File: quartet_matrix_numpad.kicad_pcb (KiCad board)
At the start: 2 copper layers, 100 x 100 mm, 62 parts, among them J2 QUARTET_RECV, SW1 Rotary_Encoder_Switch, U1 MCP23017_SS, U2 IS31FL3731-SA

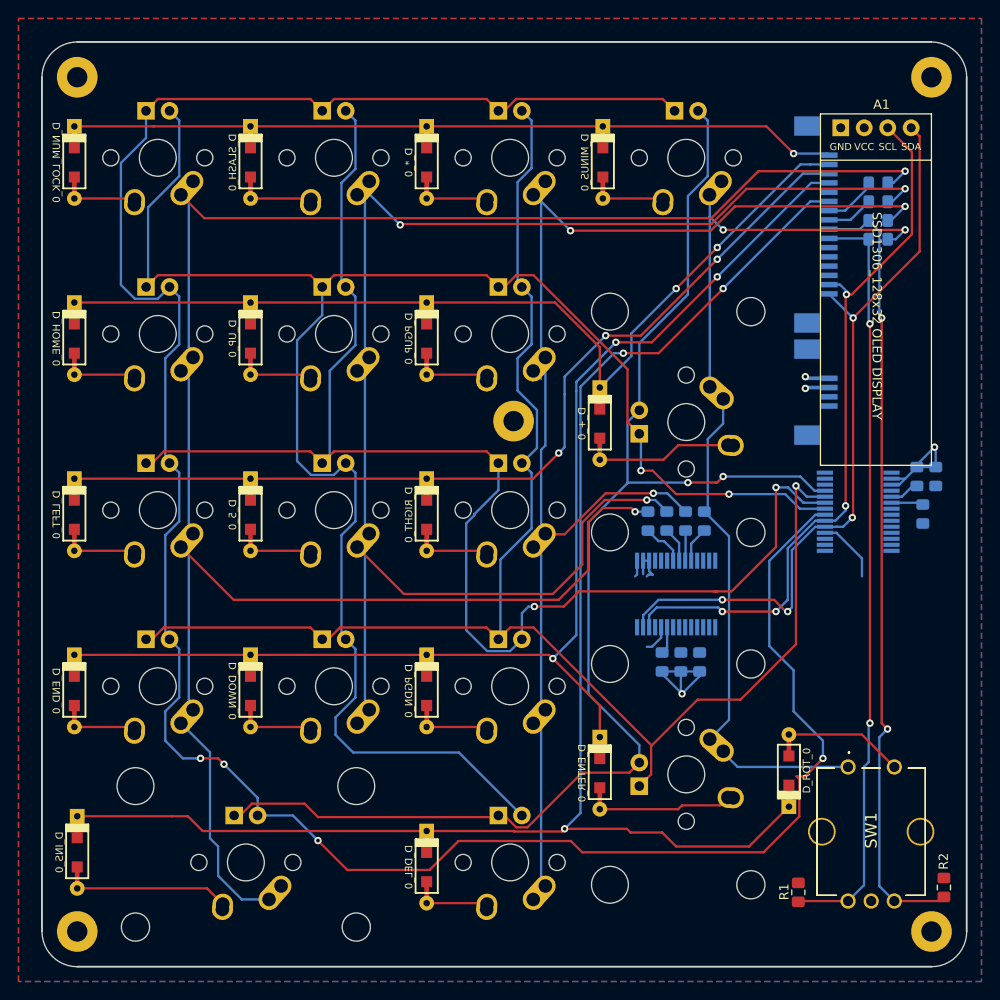
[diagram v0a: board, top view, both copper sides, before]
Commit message: Finish and route quartet mainboard
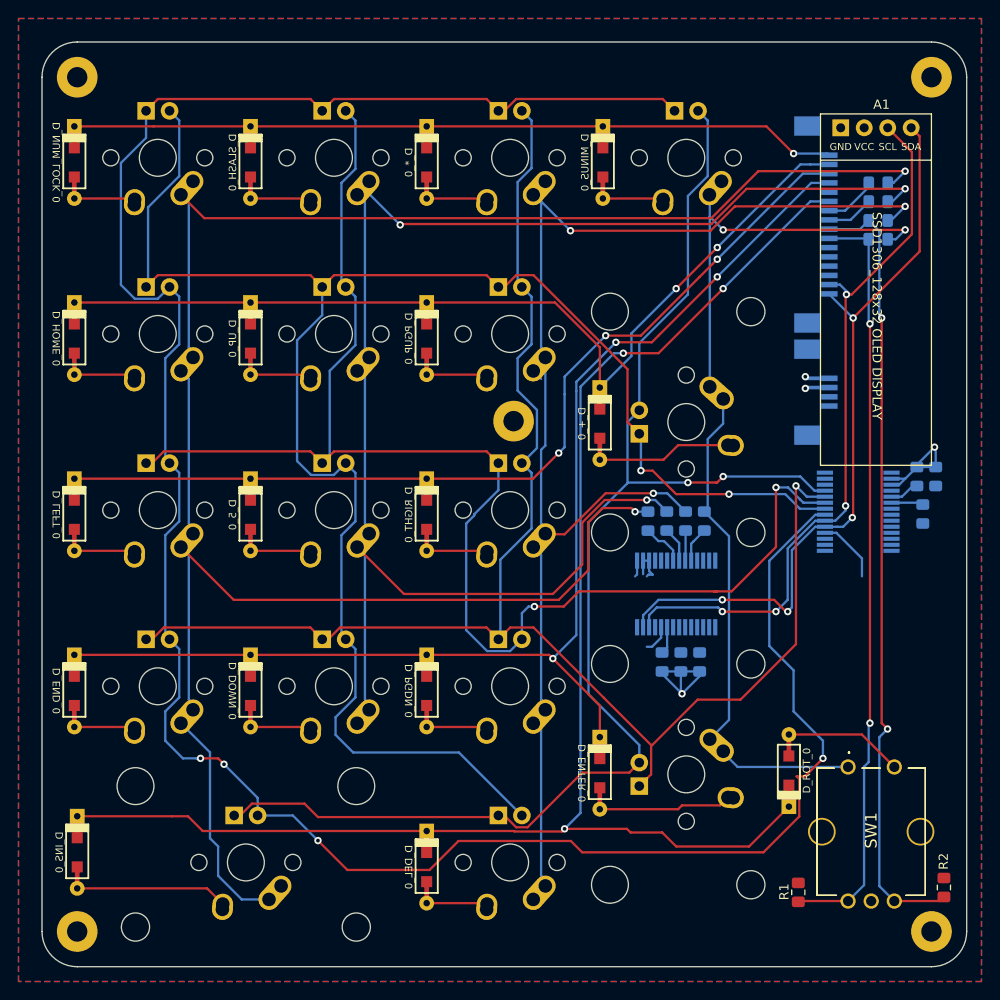
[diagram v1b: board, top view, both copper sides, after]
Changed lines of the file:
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@@
       (net 17 "Net-(D_DEL_0-Pad2)"))
   )
-  (gr_arc (start 3.81 3.81) (end 3.81 0) (angle -90) (layer Edge.Cuts) (width 0.1))
-  (gr_arc (start 3.81 96.19) (end 0 96.19) (angle -90) (layer Edge.Cuts) (width 0.1))
-  (gr_arc (start 96.19 96.19) (end 100 96.19) (angle 90) (layer Edge.Cuts) (width 0.1))
-  (gr_arc (start 96.19 3.81) (end 100 3.81) (angle -90) (layer Edge.Cuts) (width 0.1))
-  (gr_line (start 3.81 0) (end 96.19 0) (layer Edge.Cuts) (width 0.2))
-  (gr_line (start 100 3.81) (end 100 96.19) (layer Edge.Cuts) (width 0.2))
-  (gr_line (start 96.19 100) (end 3.81 100) (layer Edge.Cuts) (width 0.2))
-  (gr_line (start 0 96.19) (end 0 3.81) (layer Edge.Cuts) (width 0.2))
-  (gr_arc (start 91.725 0) (end 91.725 0) (angle 90) (layer Edge.Cuts) (width 0.2))
   (segment (start 9.925 16.925) (end 10.025 17.025) (width 0.25) (layer F.Cu) (net 1))
   (segment (start 3.5 16.925) (end 9.925 16.925) (width 0.25) (layer F.Cu) (net 1))
@@
     )
   )
+  (gr_line (start 3.810 0.000) (end 96.190 -0.000) (angle 90) (layer Edge.Cuts) (width 0.1))
+  (gr_line (start 100.000 3.810) (end 100.000 96.190) (angle 90) (layer Edge.Cuts) (width 0.1))
+  (gr_line (start 96.190 100.000) (end 3.810 100.000) (angle 90) (layer Edge.Cuts) (width 0.1))
+  (gr_line (start -0.000 96.190) (end 0.000 3.810) (angle 90) (layer Edge.Cuts) (width 0.1))
+  (gr_arc (start 3.810 3.810) (end 3.810 0.000) (angle -90.000) (layer Edge.Cuts) (width 0.1))
+  (gr_arc (start 3.810 96.190) (end -0.000 96.190) (angle -90.000) (layer Edge.Cuts) (width 0.1))
+  (gr_arc (start 96.190 96.190) (end 96.190 100.000) (angle -90.000) (layer Edge.Cuts) (width 0.1))
+  (gr_arc (start 96.190 3.810) (end 100.000 3.810) (angle -90.000) (layer Edge.Cuts) (width 0.1))
 )
